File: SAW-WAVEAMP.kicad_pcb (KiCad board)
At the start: 2 copper layers, 54.6 x 33 mm, 8 parts

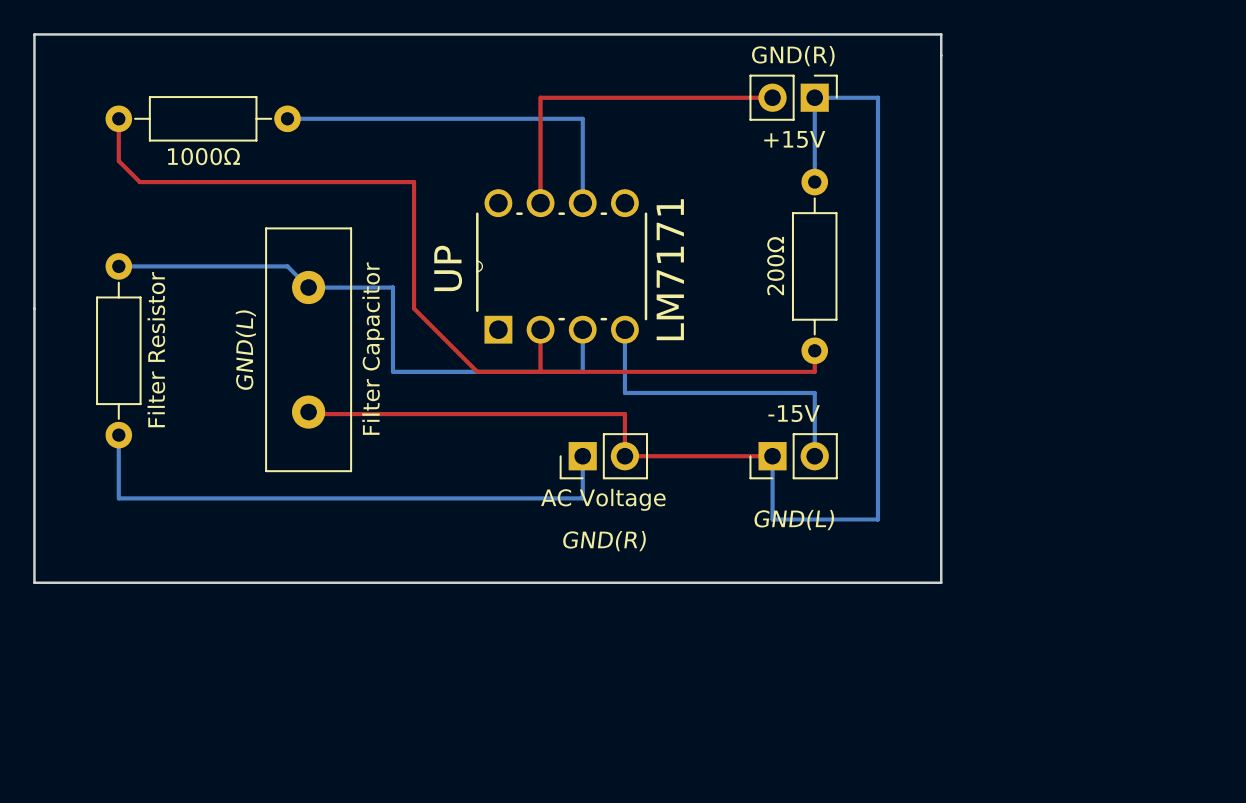
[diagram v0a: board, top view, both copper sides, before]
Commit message: Final changes for the v2.0 board (ORDERED)
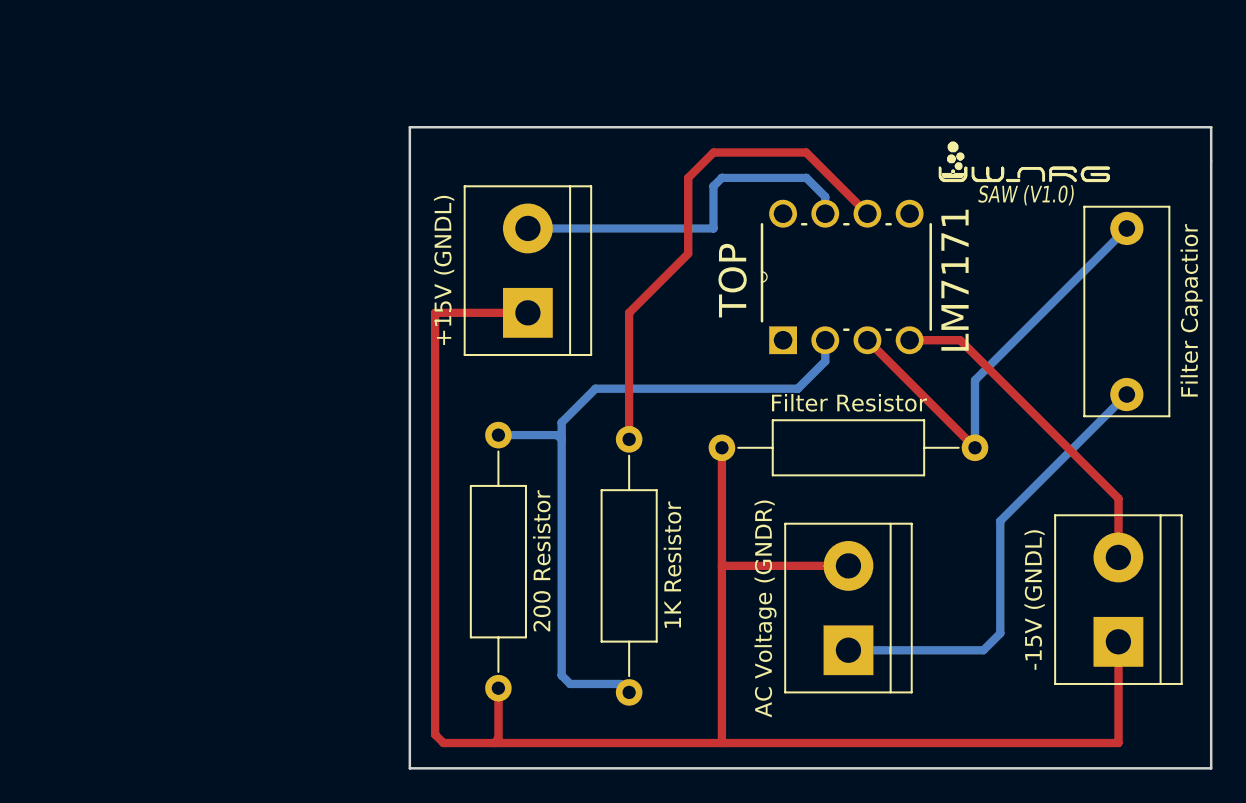
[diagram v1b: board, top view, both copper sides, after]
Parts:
- removed +15V: +15V, Pin_Headers:Pin_Header_Straight_1x02_Pitch2.54mm
- removed -15V: -15V, Pin_Headers:Pin_Header_Straight_1x02_Pitch2.54mm
- removed 1000Ω: 1K, Resistors_THT:R_Axial_DIN0207_L6.3mm_D2.5mm_P10.16mm_Horizontal
- removed 200Ω: 200, Resistors_THT:R_Axial_DIN0207_L6.3mm_D2.5mm_P10.16mm_Horizontal
- removed AC Voltage: AC Voltage Source, Pin_Headers:Pin_Header_Straight_1x02_Pitch2.54mm
- removed Filter Capacitor: Filter Capacitor, Capacitors_THT:C_Disc_D14.5mm_W5.0mm_P7.50mm
- removed the Filter Resistor at (120.7, 102.9)
- removed UP: LM7171, LM7171BIN:DIP254P762X508-8
- added +15V (GNDL): +15V, TerminalBlock:TerminalBlock_bornier-2_P5.08mm, F.Cu at (145.3, 105.7)
- added -15V (GNDL): -15V, TerminalBlock:TerminalBlock_bornier-2_P5.08mm, F.Cu at (180.8, 125.5)
- added 1K Resistor: 1K, Resistors_THT:R_Axial_DIN0309_L9.0mm_D3.2mm_P15.24mm_Horizontal, F.Cu at (151.4, 113.3)
- added 200 Resistor: 200, Resistors_THT:R_Axial_DIN0309_L9.0mm_D3.2mm_P15.24mm_Horizontal, F.Cu at (143.5, 113.0)
- added ?: , Sine-Wave-Amplifier-UWNRG-SAW:UWNRG-logo, F.Cu at (168.7, 95.0)
- added AC Voltage (GNDR): AC Voltage Source, TerminalBlock:TerminalBlock_bornier-2_P5.08mm, F.Cu at (164.6, 126.0)
- added Filter Capactior: Filter Capacitor, Capacitors_THT:C_Disc_D12.5mm_W5.0mm_P10.00mm, F.Cu at (181.4, 100.6)
- added Filter Resistor: Filter Resistor, Resistors_THT:R_Axial_DIN0309_L9.0mm_D3.2mm_P15.24mm_Horizontal, F.Cu at (157.0, 113.8)
- added TOP: LM7171, LM7171BIN:DIP254P762X508-8, F.Cu at (168.3, 99.7)
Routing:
- net Net-(J1-Pad1): track 34.3 -> 0.00 mm
- net GND: track 75.0 -> 107.2 mm, vias 2 -> 0
- net Net-(C1-Pad2): track 0.00 -> 27.1 mm, vias 0 -> 1
- net Net-(R1-Pad1): track 58.0 -> 42.3 mm, vias 0 -> 1
- net Net-(C1-Pad1): track 36.1 -> 26.2 mm
- net Net-(R2-Pad1): track 22.9 -> 30.2 mm, vias 0 -> 1
- net Net-(J3-Pad2): track 20.3 -> 22.1 mm
- net Net-(J2-Pad2): track 19.0 -> 20.1 mm
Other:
- board size 54.6 x 33 mm -> 48.3 x 38.6 mm
- board text added: "SAW (V1.0)"
- board text removed: "GND(L)"
- board text removed: "GND(R)"
